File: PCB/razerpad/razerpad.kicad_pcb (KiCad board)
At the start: 2 copper layers, 79.9 x 69.1 mm, 11 parts, among them SW1 SW_Push, SW2 SW_Push, SW3 SW_Push, SW4 RotaryEncoder_Switch, SW5 SW_Push, SW6 SW_Push, SW7 SW_Push, SW8 SW_Push, SW9 SW_Push, U1 XIAO-RP2040-DIP

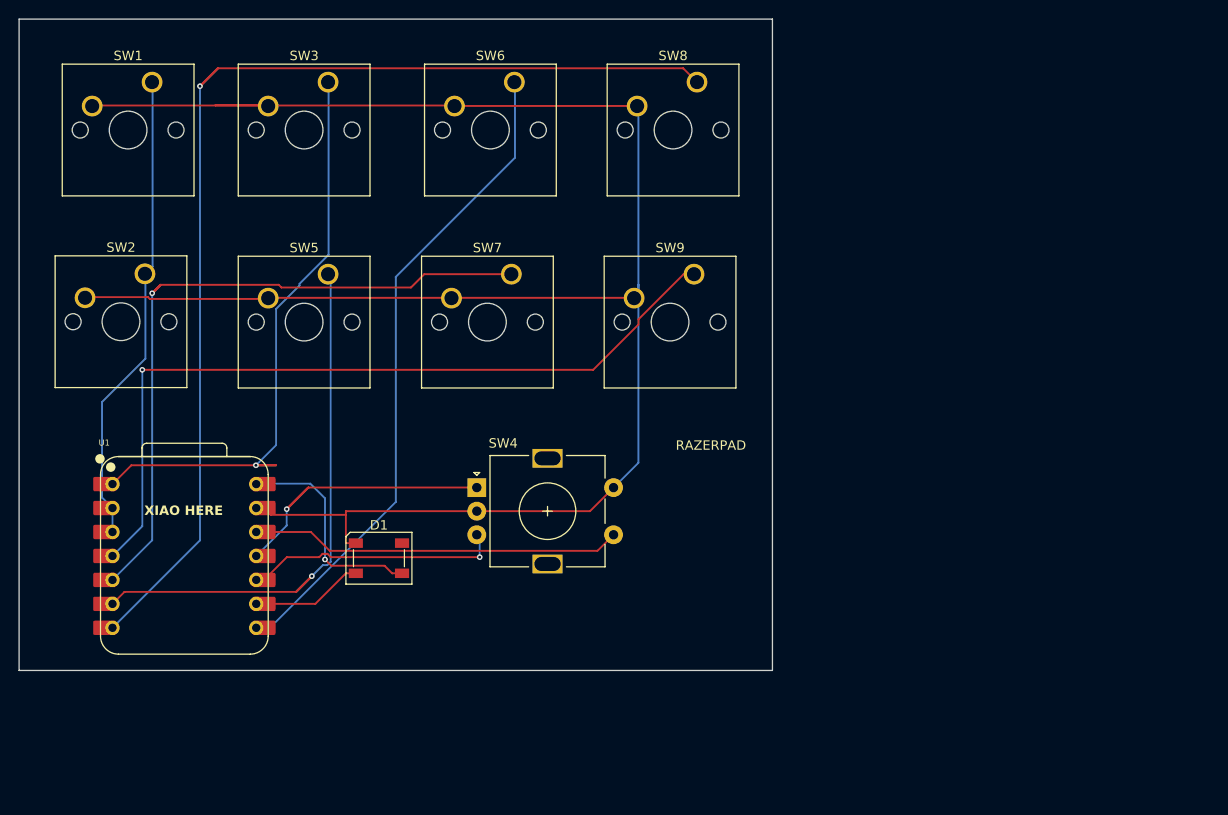
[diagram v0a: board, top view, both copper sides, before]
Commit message: alright
Signed-off-by: Shubh <shubhisroking@proton.me>
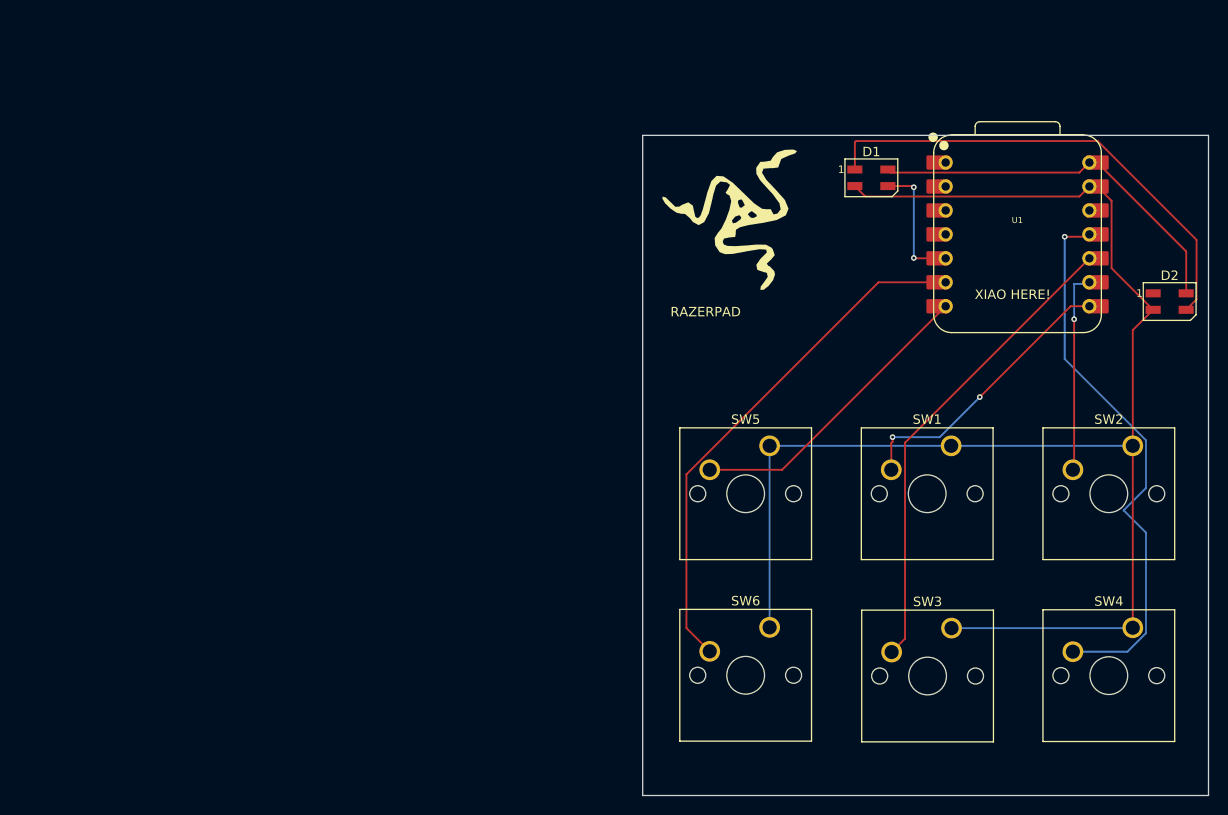
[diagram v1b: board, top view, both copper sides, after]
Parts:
- removed SW7, SW8, SW9: SW_Push, Button_Switch_Keyboard:SW_Cherry_MX_1.00u_PCB
- added D2: SK6812MINI, LED_SMD:LED_SK6812MINI_PLCC4_3.5x3.5mm_P1.75mm, F.Cu at (174.4, 80.1)
- added G***: LOGO, LOGO, F.Cu at (128.3, 71.6)
- D1: value SK6812 -> SK6812MINI; footprint LED_SMD:LED_SK6812_PLCC4_5.0x5.0mm_P3.2mm -> LED_SMD:LED_SK6812MINI_PLCC4_3.5x3.5mm_P1.75mm
- SW4: value RotaryEncoder_Switch -> SW_Push; footprint Rotary_Encoder:RotaryEncoder_Alps_EC11E-Switch_Vertical_H20mm -> Button_Switch_Keyboard:SW_Cherry_MX_1.00u_PCB
- U1: footprint Seeed Studio XIAO Series Library:XIAO-RP2040-DIP -> OPL:XIAO-RP2040-DIP
- moved SW2 106.3 mm to (170.5, 95.4)
- moved U1 94.7 mm to (158.3, 73.0)
- moved SW1 93.1 mm to (151.3, 95.4)
- moved SW3 87.9 mm to (151.3, 114.7)
- moved SW4 71.1 mm to (170.5, 114.7)
- moved D1 66.0 mm to (142.8, 67.0)
- moved SW6 63.8 mm to (132.0, 114.7)
- moved SW5 50.2 mm to (132.0, 95.4)
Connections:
- D1 pad 1: GND -> Net-(D1-DOUT)
- D1 pad 2: Net-(D1-DIN) -> GND
- D1 pad 3: +5V -> Net-(D1-DIN)
- D1 pad 4: unconnected-(D1-DOUT-Pad4) -> +5V
- SW1 pad 1: Net-(U1-GPIO27/ADC1/A1) -> GND
- SW1 pad 2: GND -> Net-(U1-GPIO1/RX)
- SW2 pad 1: Net-(U1-GPIO27/ADC1/A1) -> GND
- SW2 pad 2: GND -> Net-(U1-GPIO2/SCK)
- SW3 pad 1: Net-(U1-GPIO26/ADC0/A0) -> GND
- SW3 pad 2: GND -> Net-(U1-GPIO4/MISO)
- SW5 pad 1: Net-(U1-GPIO7/SCL) -> GND
- SW5 pad 2: GND -> Net-(U1-GPIO0/TX)
- SW6 pad 1: Net-(U1-GPIO1/RX) -> GND
- SW6 pad 2: GND -> Net-(U1-GPIO7/SCL)
- U1 pad 1: Net-(U1-GPIO26/ADC0/A0) -> unconnected-(U1-GPIO26/ADC0/A0-Pad1)
- U1 pad 12: Net-(U1-3V3) -> unconnected-(U1-3V3-Pad12)
- U1 pad 2: Net-(U1-GPIO27/ADC1/A1) -> unconnected-(U1-GPIO27/ADC1/A1-Pad2)
- U1 pad 3: Net-(U1-GPIO27/ADC1/A1) -> unconnected-(U1-GPIO28/ADC2/A2-Pad3)
- U1 pad 4: Net-(U1-GPIO29/ADC3/A3) -> unconnected-(U1-GPIO29/ADC3/A3-Pad4)
- U1 pad 5: Net-(U1-GPIO6/SDA) -> Net-(D1-DIN)
- U1 pad 9: Net-(D1-DIN) -> Net-(U1-GPIO2/SCK)
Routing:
- net Net-(U1-GPIO0/TX): track 126.9 -> 32.2 mm, vias 1 -> 0
- net Net-(U1-GPIO29/ADC3/A3): track 84.9 -> 0.00 mm, vias 1 -> 0
- net Net-(U1-GPIO6/SDA): track 77.2 -> 0.00 mm, vias 1 -> 0
- net Net-(U1-GPIO26/ADC0/A0): track 69.3 -> 0.00 mm, vias 1 -> 0
- net GND: track 208.8 -> 153.7 mm
- net Net-(U1-GPIO27/ADC1/A1): track 52.1 -> 0.00 mm
- net Net-(D1-DOUT): track 0.00 -> 51.4 mm
- net Net-(U1-GPIO1/RX): track 70.9 -> 30.1 mm, vias 0 -> 2
- net Net-(U1-3V3): track 39.4 -> 0.00 mm
- net Net-(U1-GPIO4/MISO): track 27.5 -> 50.4 mm, vias 1 -> 0
- net Net-(U1-GPIO2/SCK): track 0.00 -> 21.5 mm, vias 0 -> 1
- net Net-(U1-GPIO3/MOSI): track 41.2 -> 58.9 mm
- net +5V: track 24.0 -> 39.7 mm, vias 1 -> 0
- net Net-(U1-GPIO7/SCL): track 65.9 -> 55.7 mm, vias 1 -> 0
- net Net-(D1-DIN): track 11.9 -> 12.9 mm, vias 0 -> 2
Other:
- board size 79.9 x 69.1 mm -> 60 x 70 mm
- board text added: "XIAO HERE!"
- board text removed: "XIAO HERE"
